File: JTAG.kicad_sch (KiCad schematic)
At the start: 7 parts, among them J2 JTAG_HEADER, J3 JTAG_HEADER

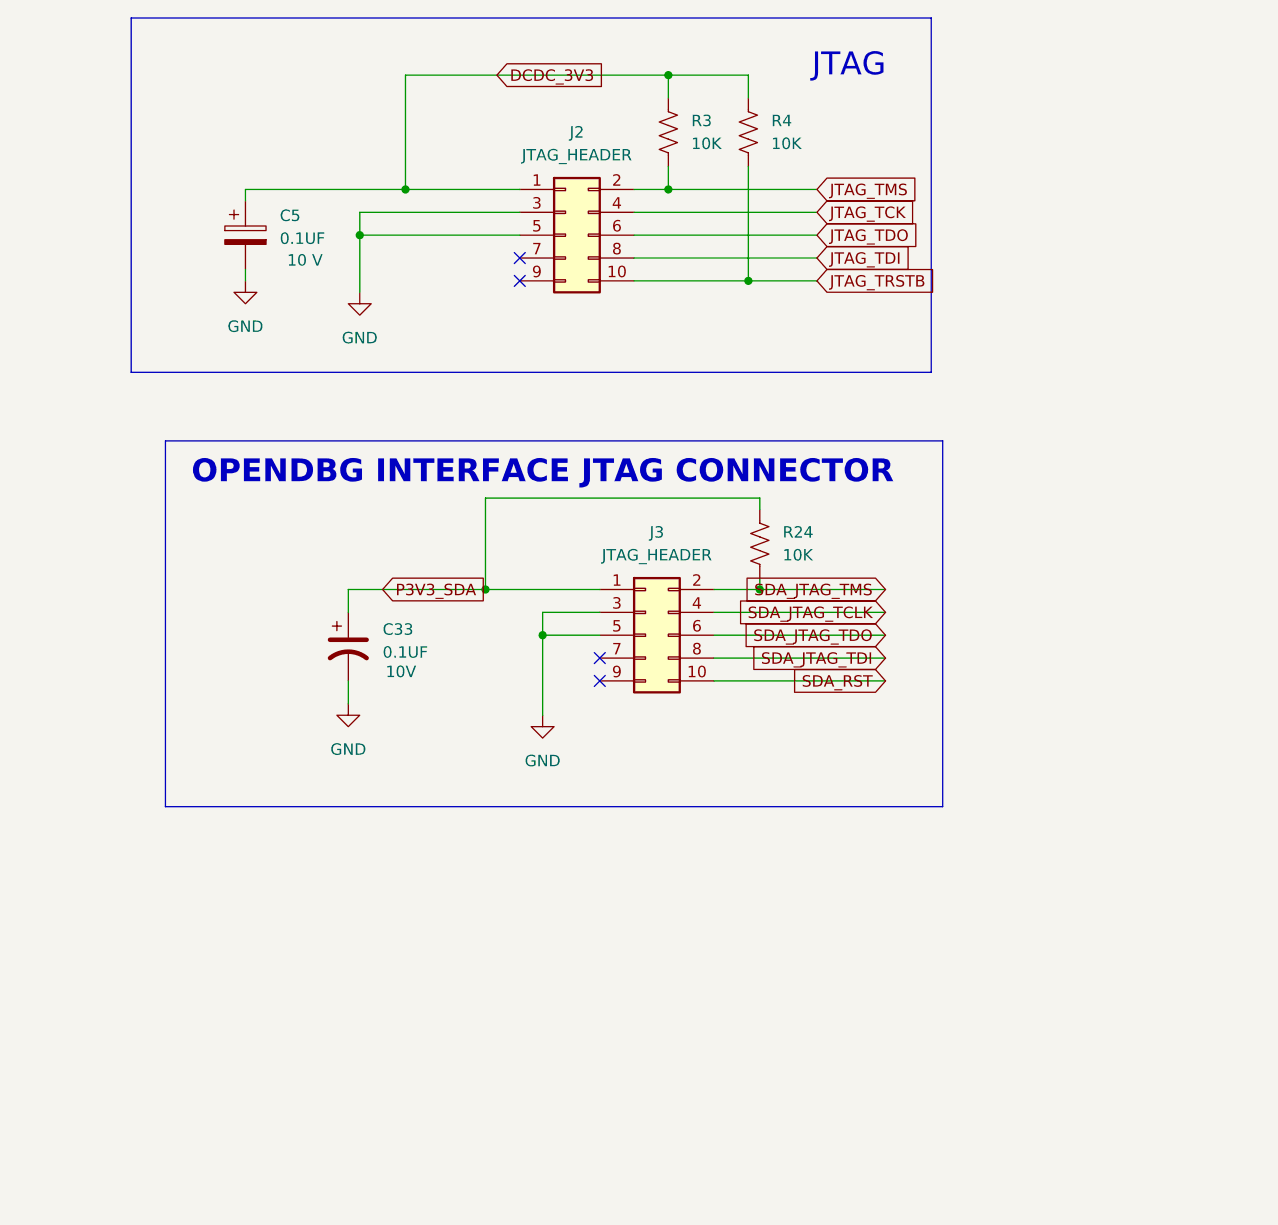
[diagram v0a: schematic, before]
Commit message: add some revision
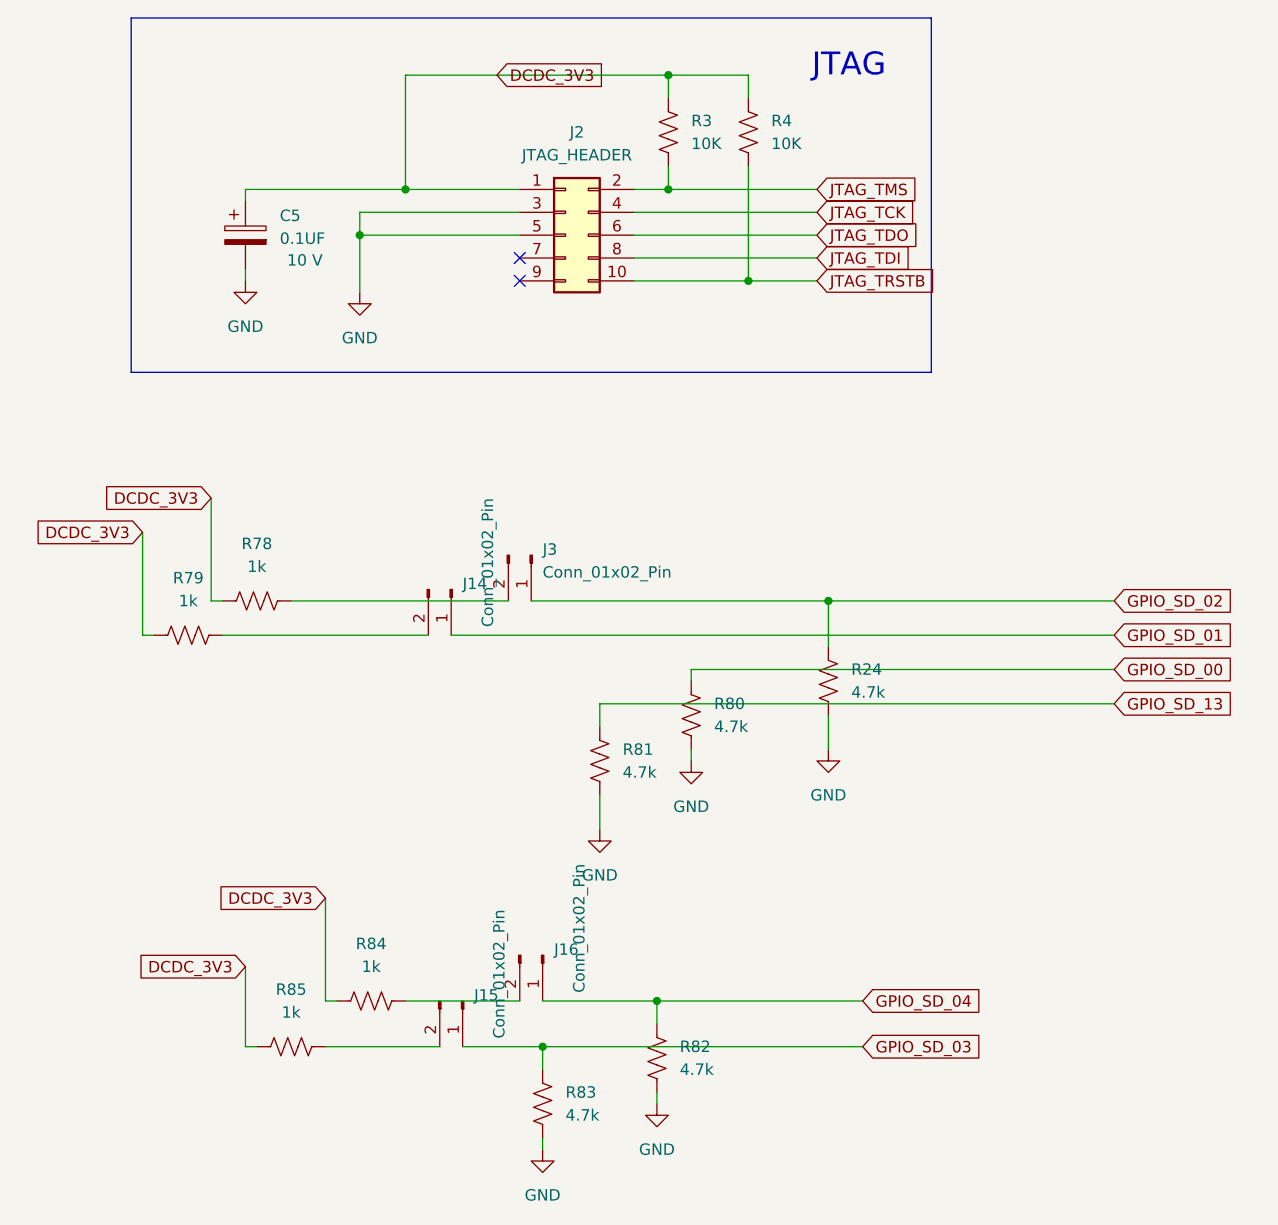
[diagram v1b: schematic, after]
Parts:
- removed C33: 0.1UF, Capacitor_SMD:C_0402_1005Metric, symbol Device:C_Polarized_US
- removed J3: JTAG_HEADER, symbol Connector_Generic:Conn_02x05_Odd_Even
- added J14, J15, J16, J3: Conn_01x02_Pin, symbol Connector:Conn_01x02_Pin
- added R78, R79, R84, R85: 1k, symbol Device:R_US
- added R80, R81, R82, R83: 4.7k, symbol Device:R_US
- R24: value 10K -> 4.7k; footprint Resistor_SMD:R_0402_1005Metric -> (none)
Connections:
- net P3V3_SDA is gone; now on net GND: R24.2
- net DCDC_3V3: now also R78.1, R79.1, R84.1, R85.1
- net GND: now also R80.2, R81.2, R82.2, R83.2
- net SDA_JTAG_TMS renamed GPIO_SD_02
- net GPIO_SD_02: now also J3.1 (Pin_1)
- new net: J16.2 (Pin_2), R84.2
- new net: J14.2 (Pin_2), R79.2
- new net: J15.2 (Pin_2), R85.2
- new net: J3.2 (Pin_2), R78.2
- new net GPIO_SD_00: R80.1
- new net GPIO_SD_01: J14.1 (Pin_1)
- new net GPIO_SD_03: J15.1 (Pin_1), R83.1
- new net GPIO_SD_04: J16.1 (Pin_1), R82.1
- new net GPIO_SD_13: R81.1
- no-connect marks 4 -> 2
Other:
- note removed: "OPENDBG INTERFACE JTAG CONNECTOR"
